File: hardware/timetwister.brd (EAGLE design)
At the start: 19.6 x 100.1 mm, 41 parts, among them IC1 PIC16F1825SO14, IC3 LM358D

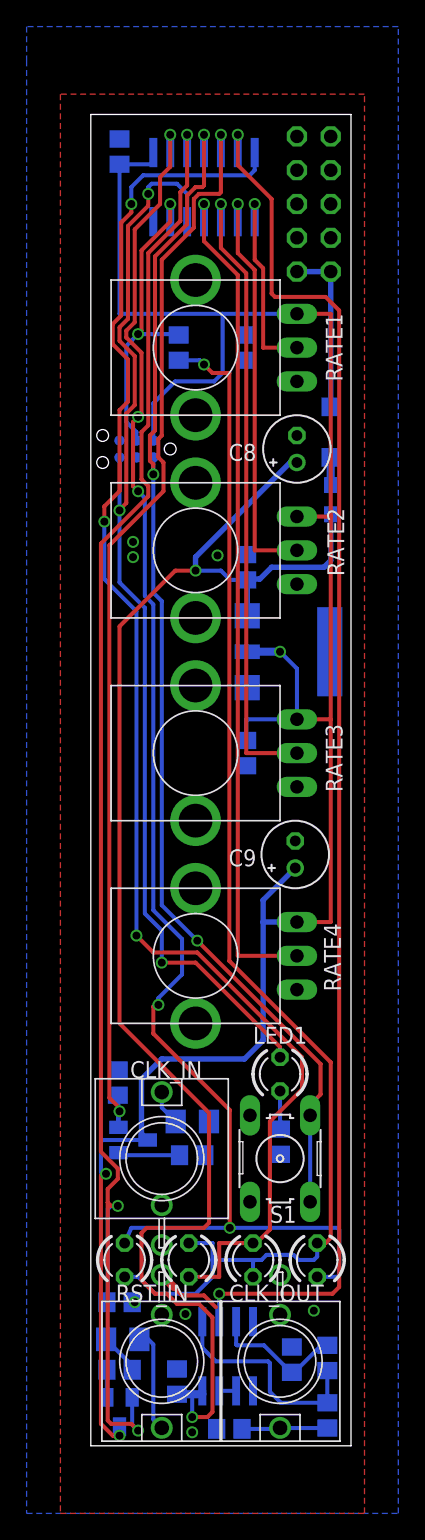
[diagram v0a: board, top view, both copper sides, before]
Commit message: sas
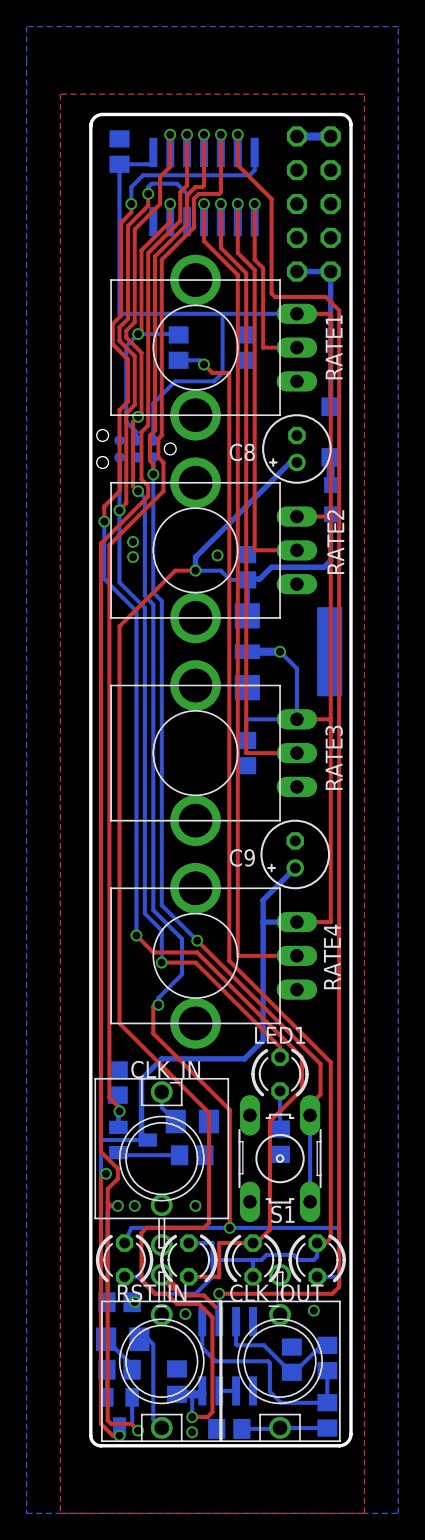
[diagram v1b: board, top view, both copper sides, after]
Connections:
- new net N$12: POWER.10, POWER.9
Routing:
- net N$12: track 0.00 -> 2.54 mm
- net GND: vias 7 -> 9
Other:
- outline, holes or cut-outs redrawn
- board text added: "2022/hotchk155"
- board text added: "DICKY TICKER V1"
- board text removed: "TIME TWISTER v1"
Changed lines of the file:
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@@
 <layer number="20" name="Dimension" color="15" fill="1" visible="yes" active="yes"/>
 <layer number="21" name="tPlace" color="7" fill="1" visible="yes" active="yes"/>
-<layer number="22" name="bPlace" color="7" fill="1" visible="yes" active="yes"/>
+<layer number="22" name="bPlace" color="7" fill="1" visible="no" active="yes"/>
 <layer number="23" name="tOrigins" color="15" fill="1" visible="yes" active="yes"/>
-<layer number="24" name="bOrigins" color="15" fill="1" visible="yes" active="yes"/>
+<layer number="24" name="bOrigins" color="15" fill="1" visible="no" active="yes"/>
 <layer number="25" name="tNames" color="7" fill="1" visible="yes" active="yes"/>
-<layer number="26" name="bNames" color="7" fill="1" visible="yes" active="yes"/>
+<layer number="26" name="bNames" color="7" fill="1" visible="no" active="yes"/>
 <layer number="27" name="tValues" color="7" fill="1" visible="yes" active="yes"/>
-<layer number="28" name="bValues" color="7" fill="1" visible="yes" active="yes"/>
+<layer number="28" name="bValues" color="7" fill="1" visible="no" active="yes"/>
 <layer number="29" name="tStop" color="7" fill="3" visible="yes" active="yes"/>
 <layer number="30" name="bStop" color="7" fill="6" visible="yes" active="yes"/>
@@
 <layer number="49" name="Reference" color="7" fill="1" visible="yes" active="yes"/>
 <layer number="50" name="dxf" color="7" fill="1" visible="no" active="no"/>
-<layer number="51" name="tDocu" color="7" fill="1" visible="yes" active="yes"/>
+<layer number="51" name="tDocu" color="7" fill="1" visible="no" active="yes"/>
 <layer number="52" name="bDocu" color="7" fill="1" visible="yes" active="yes"/>
 <layer number="53" name="tGND_GNDA" color="7" fill="9" visible="no" active="no"/>
@@
 <board>
 <plain>
-<wire x1="3.556" y1="0" x2="23.114" y2="0" width="0" layer="20"/>
-<wire x1="23.114" y1="0" x2="23.114" y2="100.076" width="0" layer="20"/>
-<wire x1="23.114" y1="100.076" x2="3.556" y2="100.076" width="0" layer="20"/>
-<wire x1="3.556" y1="100.076" x2="3.556" y2="0" width="0" layer="20"/>
+<wire x1="3.556" y1="99.314" x2="3.556" y2="99.187" width="0" layer="20"/>
+<wire x1="3.556" y1="99.187" x2="3.556" y2="0.762" width="0" layer="20"/>
 <wire x1="17.78" y1="99.695" x2="17.78" y2="86.36" width="0.3048" layer="22"/>
 <wire x1="17.78" y1="86.36" x2="22.86" y2="86.36" width="0.3048" layer="22"/>
@@
 <text x="17.653" y="89.535" size="1.27" layer="22" font="vector" ratio="20" rot="MR270">+12</text>
 <text x="17.653" y="99.695" size="1.27" layer="22" font="vector" ratio="20" rot="MR270">-12</text>
-<text x="6.223" y="62.611" size="2.032" layer="22" font="vector" ratio="20" rot="MR270">TIME TWISTER v1</text>
+<text x="6.223" y="62.611" size="2.032" layer="22" font="vector" ratio="20" rot="MR270">DICKY TICKER V1</text>
 <wire x1="3.81" y1="77.47" x2="3.81" y2="72.39" width="0.3048" layer="22"/>
 <wire x1="3.81" y1="72.39" x2="10.16" y2="72.39" width="0.3048" layer="22"/>
 <wire x1="10.16" y1="72.39" x2="10.16" y2="77.47" width="0.3048" layer="22"/>
 <wire x1="10.16" y1="77.47" x2="3.81" y2="77.47" width="0.3048" layer="22"/>
+<text x="8.128" y="62.103" size="1.27" layer="22" font="vector" ratio="20" rot="MR270">2022/hotchk155</text>
+<wire x1="3.556" y1="99.187" x2="4.445" y2="100.076" width="0.254" layer="20" curve="-90"/>
+<wire x1="4.445" y1="100.076" x2="22.352" y2="100.076" width="0.254" layer="20"/>
+<wire x1="22.352" y1="100.076" x2="23.114" y2="99.314" width="0.254" layer="20" curve="-90"/>
+<wire x1="23.114" y1="99.314" x2="23.114" y2="0.889" width="0.254" layer="20"/>
+<wire x1="23.114" y1="0.889" x2="22.225" y2="0" width="0.254" layer="20" curve="-90"/>
+<wire x1="22.225" y1="0" x2="4.318" y2="0" width="0.254" layer="20"/>
+<wire x1="4.318" y1="0" x2="3.556" y2="0.762" width="0.254" layer="20" curve="-90"/>
+<wire x1="3.556" y1="0.762" x2="3.556" y2="99.314" width="0.254" layer="20"/>
 </plain>
 <attributes>
@@
 <via x="6.858" y="10.795" extent="1-16" drill="0.6"/>
 <wire x1="8.89" y1="12.85" x2="8.89" y2="12.827" width="0.6096" layer="1"/>
-<wire x1="8.89" y1="12.827" x2="9.779" y2="11.938" width="0.6096" layer="1"/>
 <via x="11.176" y="1.016" extent="1-16" drill="0.6"/>
 <wire x1="9.779" y1="11.938" x2="10.414" y2="11.303" width="0.3048" layer="1"/>
@@
 <via x="6.731" y="66.802" extent="1-16" drill="0.6"/>
 <via x="13.081" y="66.929" extent="1-16" drill="0.6"/>
+<wire x1="8.89" y1="12.827" x2="9.779" y2="11.938" width="0.6096" layer="1"/>
+<via x="11.43" y="18.034" extent="1-16" drill="0.6"/>
+<via x="6.858" y="18.034" extent="1-16" drill="0.6"/>
 </signal>
 <signal name="CLOCK_OUT">
@@
 <wire x1="6.096" y1="12.7" x2="7.112" y2="12.7" width="0.3048" layer="16"/>
 <wire x1="7.112" y1="12.7" x2="8.382" y2="11.43" width="0.3048" layer="16"/>
-<wire x1="8.382" y1="11.43" x2="11.303" y2="11.43" width="0.3048" layer="16"/>
+<wire x1="8.382" y1="11.43" x2="11.43" y2="11.43" width="0.3048" layer="16"/>
 <wire x1="10.922" y1="15.24" x2="12.7" y2="15.24" width="0.3048" layer="16"/>
 <wire x1="12.7" y1="15.24" x2="12.7" y2="13.97" width="0.3048" layer="16"/>
@@
 <wire x1="18.796" y1="14.351" x2="19.177" y2="13.97" width="0.3048" layer="16"/>
 <wire x1="19.177" y1="13.97" x2="20.32" y2="13.97" width="0.3048" layer="16"/>
-<wire x1="11.303" y1="11.43" x2="11.43" y2="11.43" width="0" layer="19" extent="16-16"/>
 </signal>
 <signal name="LED_COM">
@@
 <contactref element="C3" pad="1"/>
 <contactref element="C8" pad="+"/>
-<contactref element="L1" pad="2"/>
 <via x="11.43" y="65.786" extent="1-16" drill="0.6"/>
 <wire x1="15.475" y1="62.23" x2="15.315" y2="62.39" width="0.6096" layer="16"/>
@@
 <wire x1="11.938" y1="3.937" x2="11.176" y2="3.937" width="0.4064" layer="16"/>
 <via x="11.176" y="2.159" extent="1-16" drill="0.6"/>
-<wire x1="21.59" y1="70.02" x2="21.59" y2="66.548" width="0.4064" layer="16"/>
 <wire x1="21.59" y1="66.548" x2="21.082" y2="66.04" width="0.4064" layer="16"/>
 <wire x1="21.082" y1="66.04" x2="17.145" y2="66.04" width="0.4064" layer="16"/>
@@
 <wire x1="18.542" y1="73.914" x2="11.43" y2="66.802" width="0.4064" layer="16"/>
 <wire x1="11.43" y1="66.802" x2="11.43" y2="65.786" width="0.4064" layer="16"/>
+<contactref element="L1" pad="2"/>
+<wire x1="21.59" y1="66.548" x2="21.59" y2="70.02" width="0.4064" layer="16"/>
 </signal>
 <signal name="N$13">
 <contactref element="POWER" pad="1"/>
 <contactref element="POWER" pad="2"/>
+<wire x1="21.59" y1="88.265" x2="19.05" y2="88.265" width="0.4064" layer="16"/>
 <contactref element="D1" pad="A"/>
-<wire x1="21.59" y1="78.1" x2="21.59" y2="88.265" width="0.4064" layer="16"/>
-<wire x1="21.59" y1="88.265" x2="19.05" y2="88.265" width="0.4064" layer="16"/>
+<wire x1="21.59" y1="88.265" x2="21.59" y2="78.1" width="0.4064" layer="16"/>
 </signal>
 <signal name="N$15">
@@
 <wire x1="8.89" y1="38.735" x2="8.89" y2="36.322" width="0.3048" layer="16"/>
 </signal>
+<signal name="N$12">
+<contactref element="POWER" pad="9"/>
+<contactref element="POWER" pad="10"/>
+<wire x1="19.05" y1="98.425" x2="21.59" y2="98.425" width="0.6096" layer="16"/>
+</signal>
 </signals>
